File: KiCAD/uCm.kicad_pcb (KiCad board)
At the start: 2 copper layers, 99 x 122 mm, 102 parts, among them J1 5V_EXT, J2 3V3_EXT, P1 AREF, P10 C3SB, P11 VSel_Vlv, P13 PWR_IN, P14 X_VALVE, P17 PUMP, P24 PWR_IN, P34 VSel_Vlv2, P38 X_VALVE2, P4 ICSP, P5 FTDI, P7 GAGE_PR, P9 C3SB, Q1 BCP5416TA, Q2 BCP5416TA, Q3 BCP5416TA, Q4 BCP5416TA, SW1 Reset, SW2 INT0, SW3 INT1, U1 TXB0104D, U3 TPS62133, U4 TPS62132, U5 DS3231N, U7 ATMEGA328-AU-ND, X1 16MHz

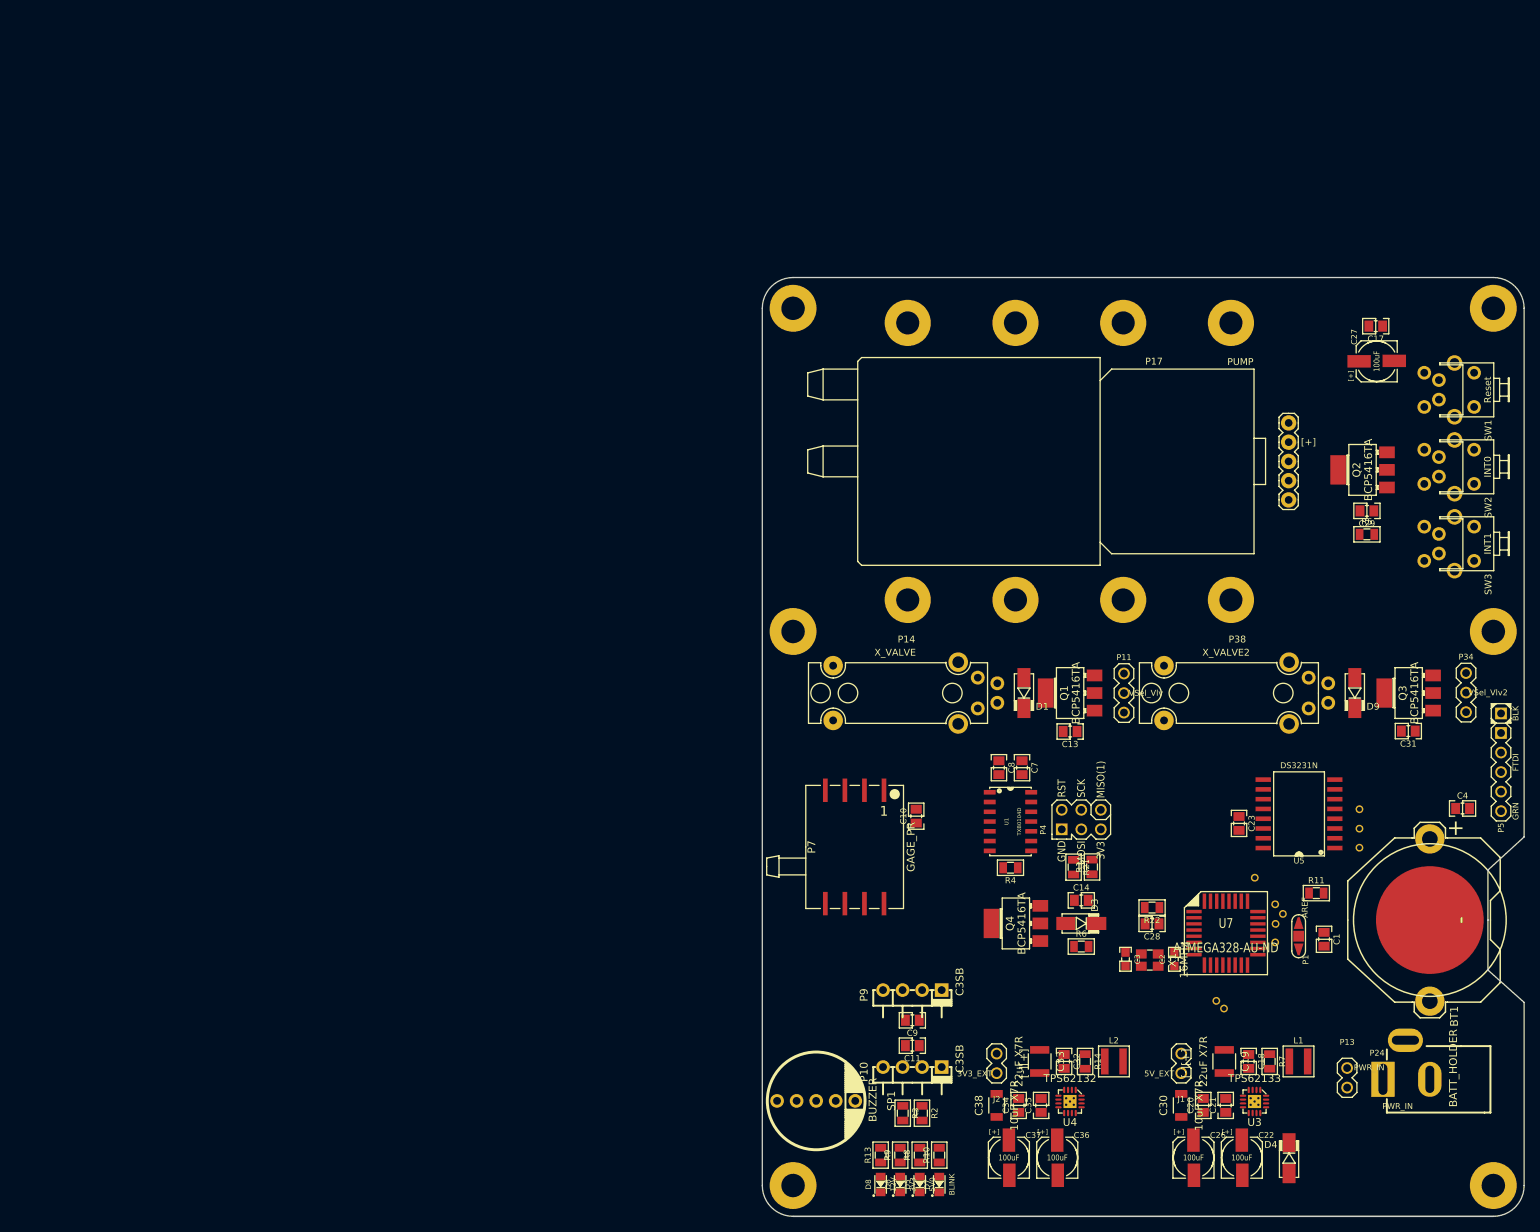
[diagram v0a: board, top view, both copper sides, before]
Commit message: layout, work in progress
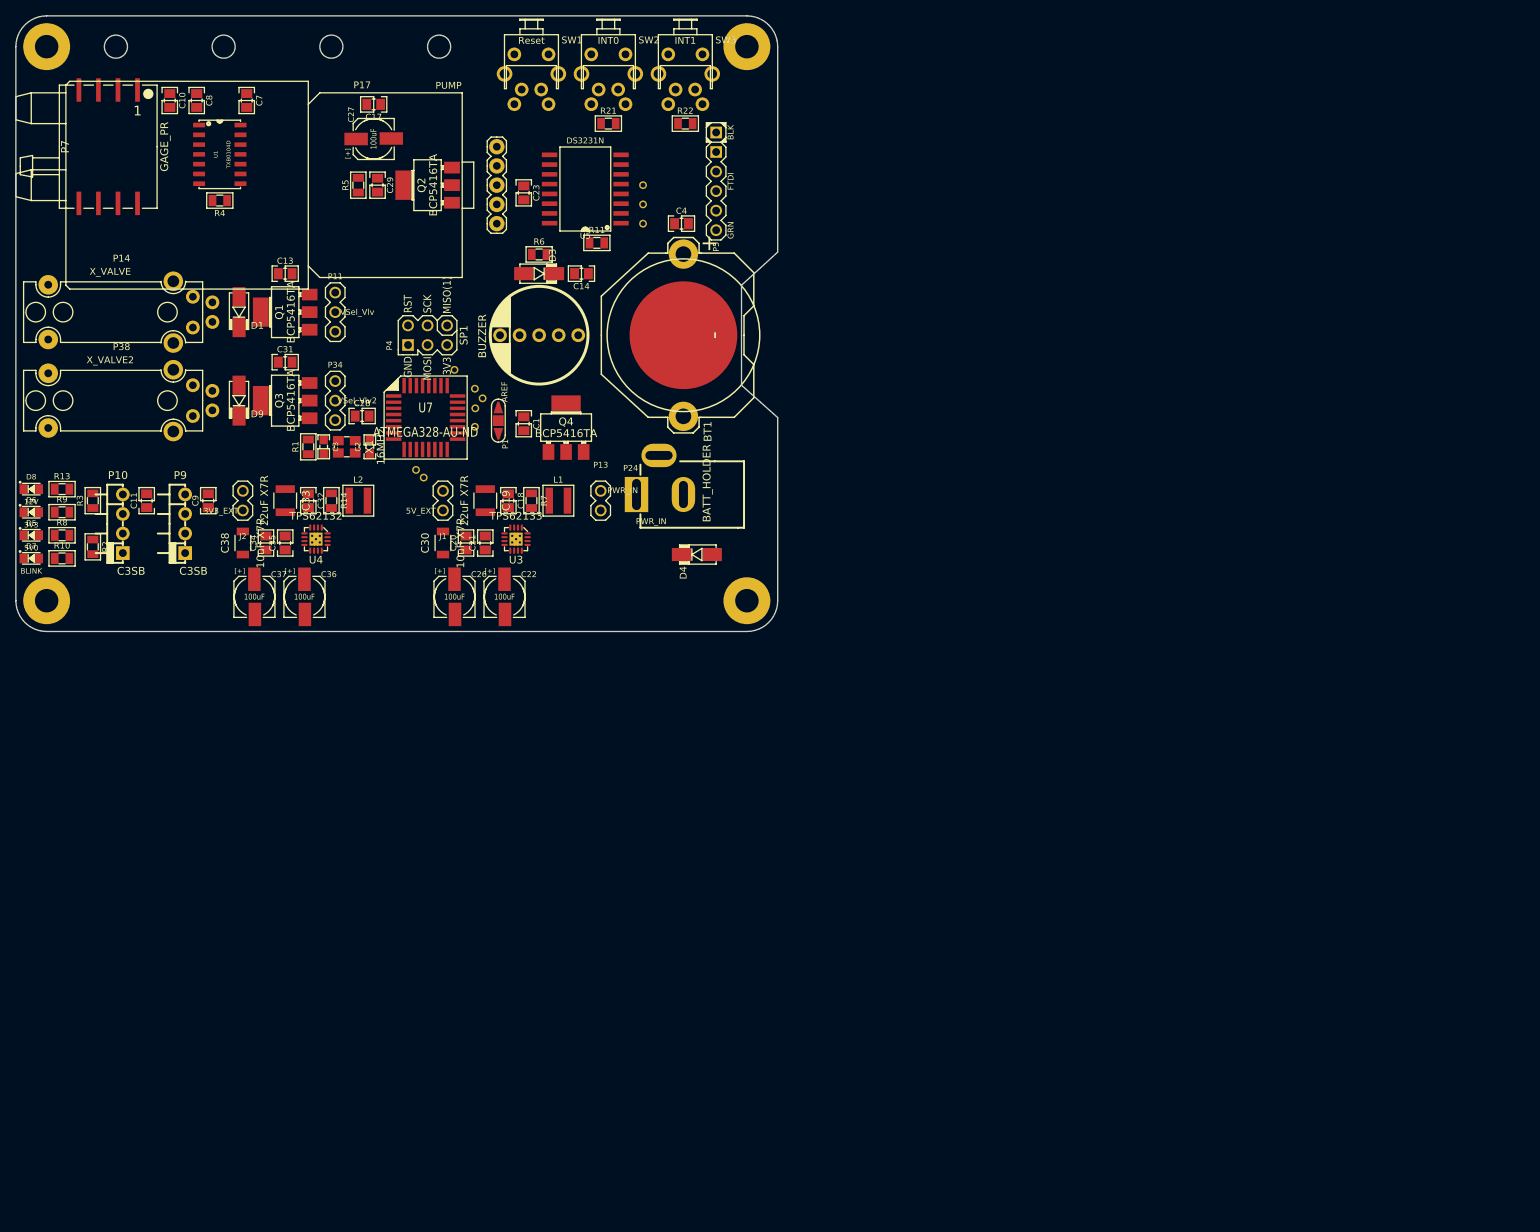
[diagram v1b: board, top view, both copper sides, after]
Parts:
- removed SC3, SC4: SCREW, uCm:vite_3mm
- P17: footprint uCm:Pump_P54E01R_02 -> uCm:Pump_P54E01R_03
- moved C31 153.6 mm to (49.0, 59.0), turned to 0 degrees
- moved P34 151.8 mm to (55.5, 64.0)
- moved Q3 150.9 mm to (49.0, 64.0)
- moved D9 149.9 mm to (43.0, 64.0)
- moved P38 149.9 mm to (37.0, 64.0)
- moved D7 143.3 mm to (16.0, 84.5), turned to 0 degrees
- moved D5 143.0 mm to (16.0, 81.5), turned to 0 degrees
- moved D6 142.8 mm to (16.0, 78.5), turned to 0 degrees
- moved D8 142.6 mm to (16.0, 75.5), turned to 0 degrees
- moved R5 138.7 mm to (58.5, 36.0), turned to 90 degrees
- moved R10 137.9 mm to (20.0, 84.5), turned to 0 degrees
- moved R8 137.5 mm to (20.0, 81.5), turned to 0 degrees
- moved R9 137.3 mm to (20.0, 78.5), turned to 0 degrees
- moved R13 137.1 mm to (20.0, 75.5), turned to 0 degrees
- moved C8 135.6 mm to (37.5, 25.0)
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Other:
- board size 99 x 122 mm -> 99 x 80 mm
- board text removed: "[+]"
- board text removed: "[+][-]"
